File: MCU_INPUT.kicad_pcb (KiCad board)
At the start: 2 copper layers, 62 x 32 mm, 32 parts, among them J1 Conn_01x04_Female, J2 Conn_01x20_Female, SW1 SW_Push, SW2 Rotary_Encoder, SW3 SW_Push, SW4 SW_Push

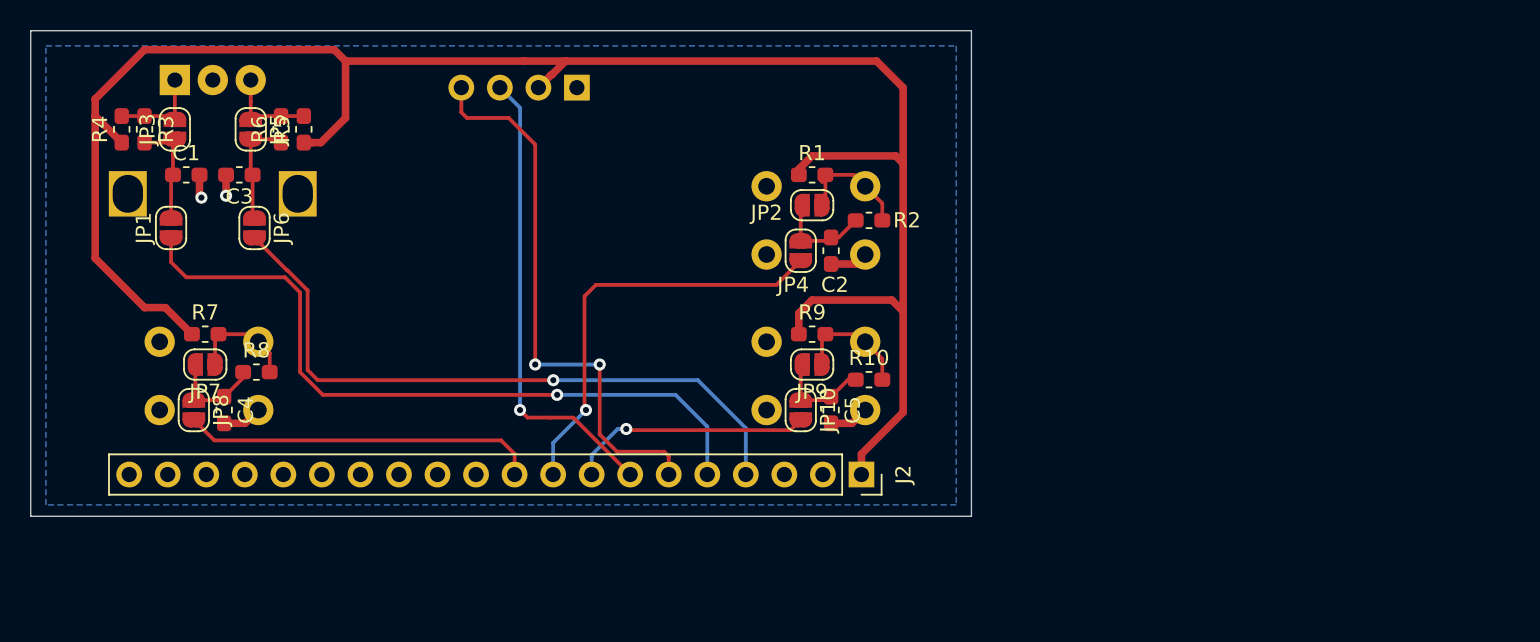
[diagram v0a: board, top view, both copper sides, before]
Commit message: ordered
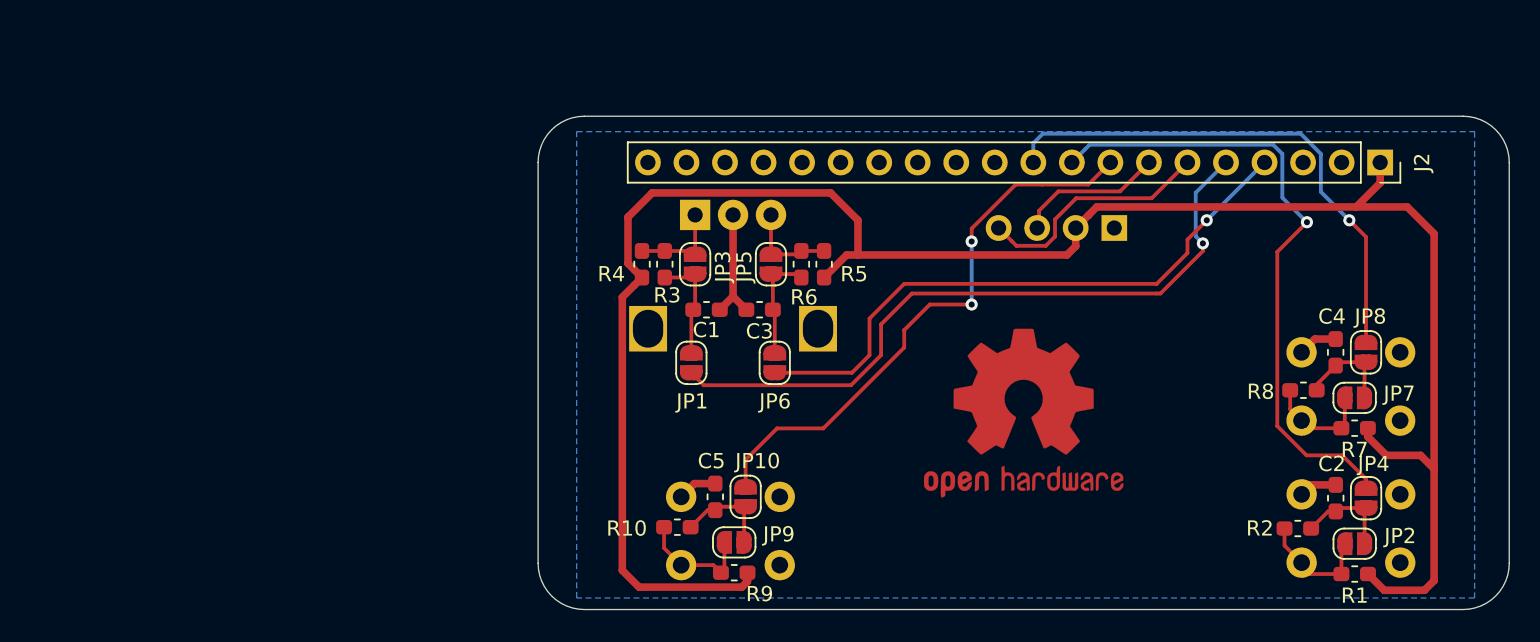
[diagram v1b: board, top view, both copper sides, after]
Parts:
- added REF**: OSHW-Logo2_14.6x12mm_Copper, Symbol:OSHW-Logo2_14.6x12mm_Copper, F.Cu at (123.4, 91.7)
- moved PB3 81.8 mm to (148.3, 87.7), turned to 180 degrees
- moved JP8 77.4 mm to (146.0, 87.7), turned to 90 degrees
- moved R7 76.0 mm to (145.3, 92.7), turned to 180 degrees
- moved JP7 75.8 mm to (145.3, 90.7), turned to 0 degrees
- moved C4 73.4 mm to (144.0, 87.7), turned to 90 degrees
- moved R8 69.0 mm to (141.9, 90.2), turned to 180 degrees
- moved PB4 44.7 mm to (148.3, 97.1), turned to 180 degrees
- moved R1 44.4 mm to (145.3, 102.3), turned to 180 degrees
- moved JP2 42.1 mm to (145.3, 100.3), turned to 0 degrees
- moved JP4 40.7 mm to (146.0, 97.3), turned to 90 degrees
- moved J2 39.9 mm to (146.9, 75.2)
- moved C2 37.0 mm to (144.0, 97.3), turned to 90 degrees
- moved OLED_IIC 36.6 mm to (129.4, 79.5)
- moved REF** 35.9 mm to (125.7, 89.2)
- moved C1 35.4 mm to (102.5, 84.9)
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- renumbered J1 to OLED_IIC, SW3 to PB3, SW1 to PB4, SW4 to PB5
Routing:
- net /PB5: track 16.1 -> 37.6 mm, vias 1 -> 2
- net /PB7: track 37.1 -> 15.9 mm, vias 2 -> 0
- net /PB6: track 30.4 -> 9.75 mm, vias 1 -> 0
- net /PB4: track 27.9 -> 41.9 mm
- net /PB3: track 23.4 -> 34.7 mm, vias 0 -> 1
- net GND: track 10.7 -> 15.6 mm, vias 2 -> 0
- net /PB9: track 43.7 -> 40.0 mm
- net VCC: track 130.7 -> 133.4 mm
- net /PB8: track 47.7 -> 45.8 mm
- net Net-(JP2-Pad1): track 8.77 -> 7.86 mm
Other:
- board size 62 x 32 mm -> 64 x 32.5 mm
